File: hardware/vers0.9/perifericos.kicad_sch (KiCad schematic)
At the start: 27 parts, among them J4 Conn_02x13_Odd_Even, J5 Teclado, J6 Encoders, U10 ULN2803A, U2 74HC595, U6 74HC165

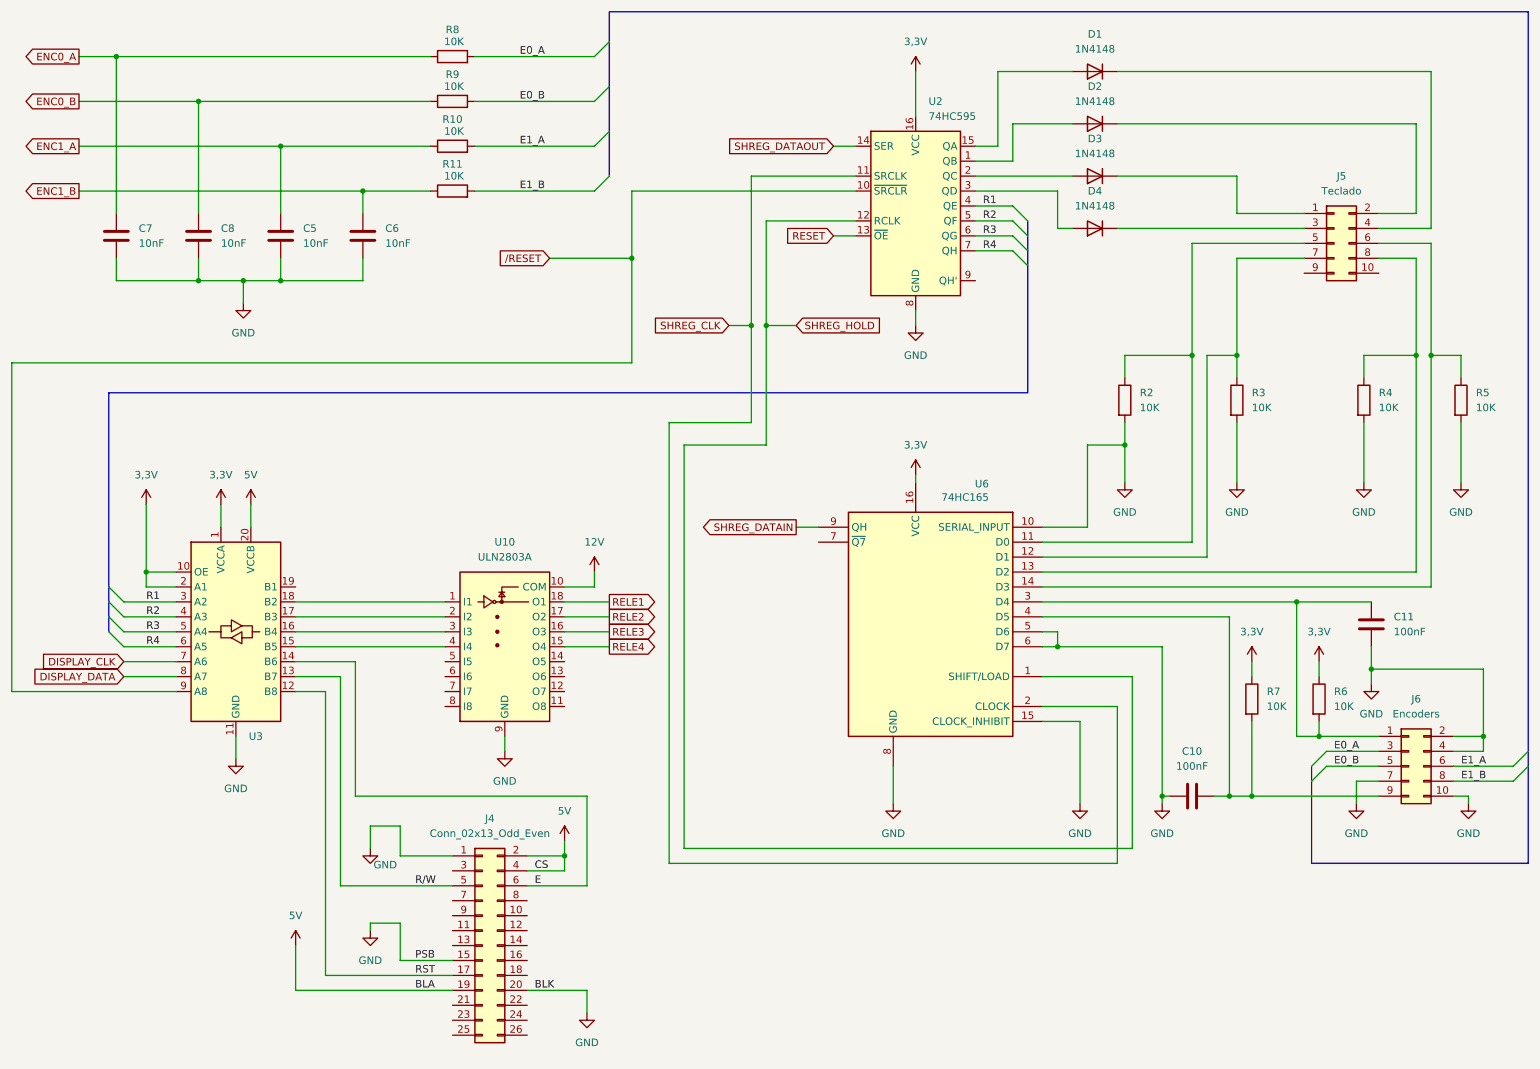
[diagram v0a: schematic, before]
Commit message: 250826-1410
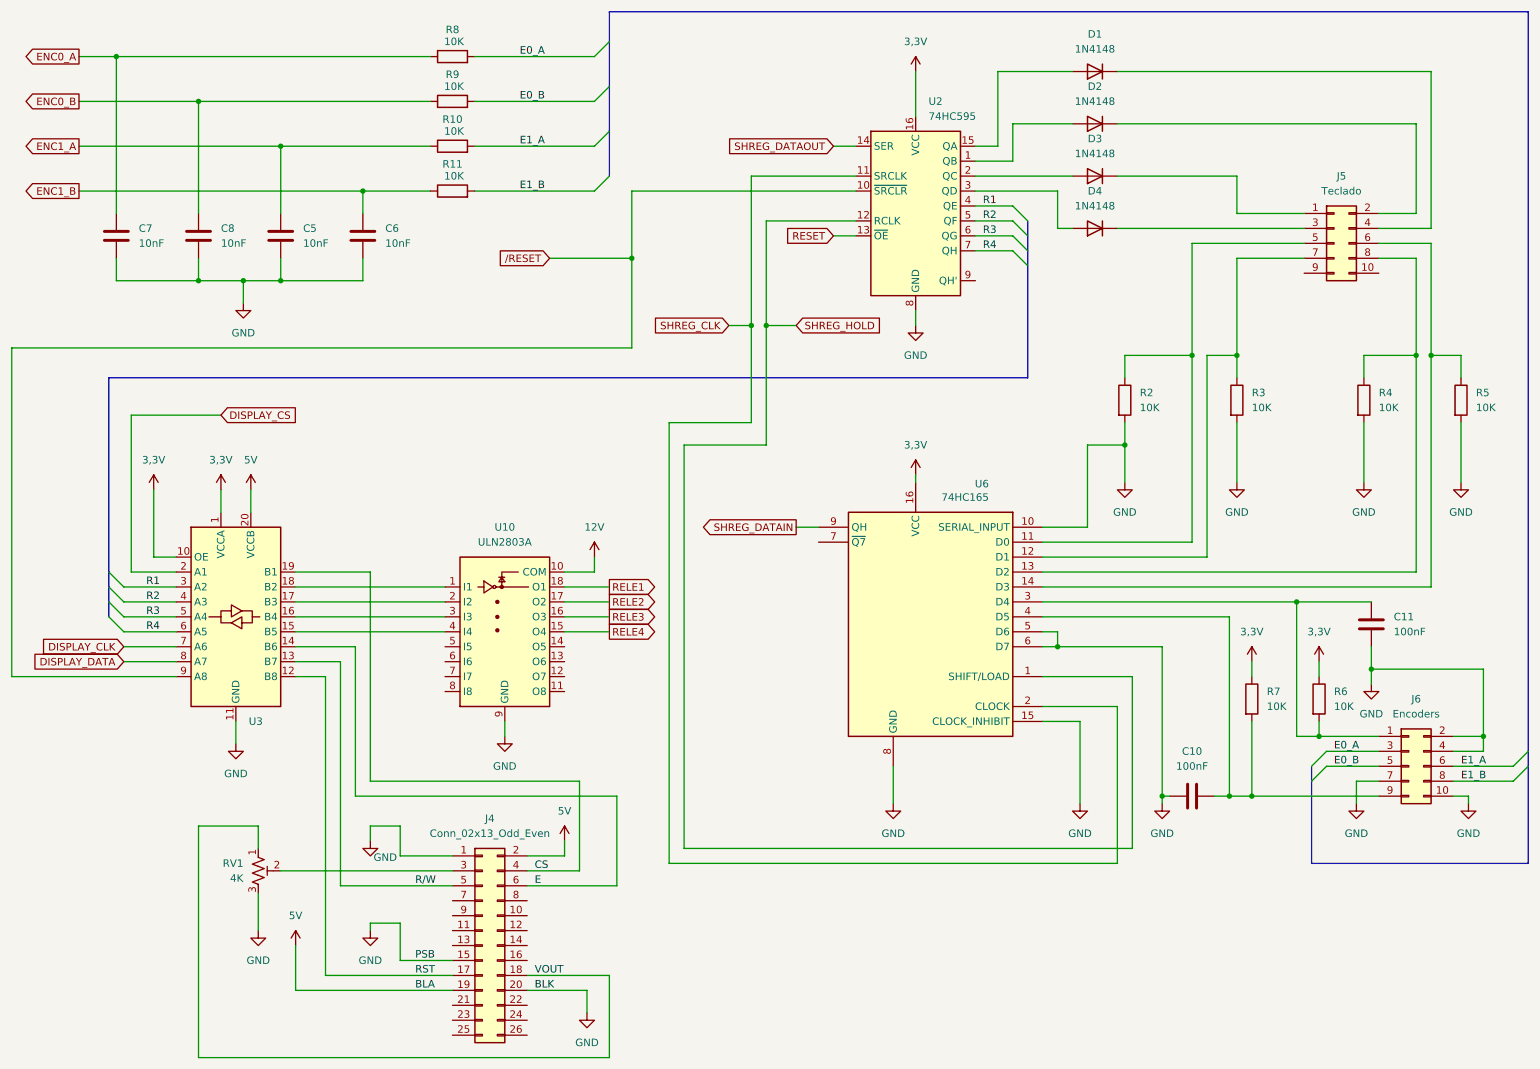
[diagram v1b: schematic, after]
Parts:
- added RV1: 4K, symbol Device:R_Potentiometer_Trim_US
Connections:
- net 3,3V: no longer U3.2 (A1)
- net 5V: no longer J4.4 (Pin_4)
- net GND: now also RV1.3
- net VOUT: now reaches J4.18 (Pin_18)
- net VOUT: now also RV1.1
- net at J4.3 (Pin_3): now also RV1.2
- net CS: now reaches U3.19 (B1)
- net CS: now also J4.4 (Pin_4)
- new net DISPLAY_CS: U3.2 (A1)
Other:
- moved on the sheet: U10, U3

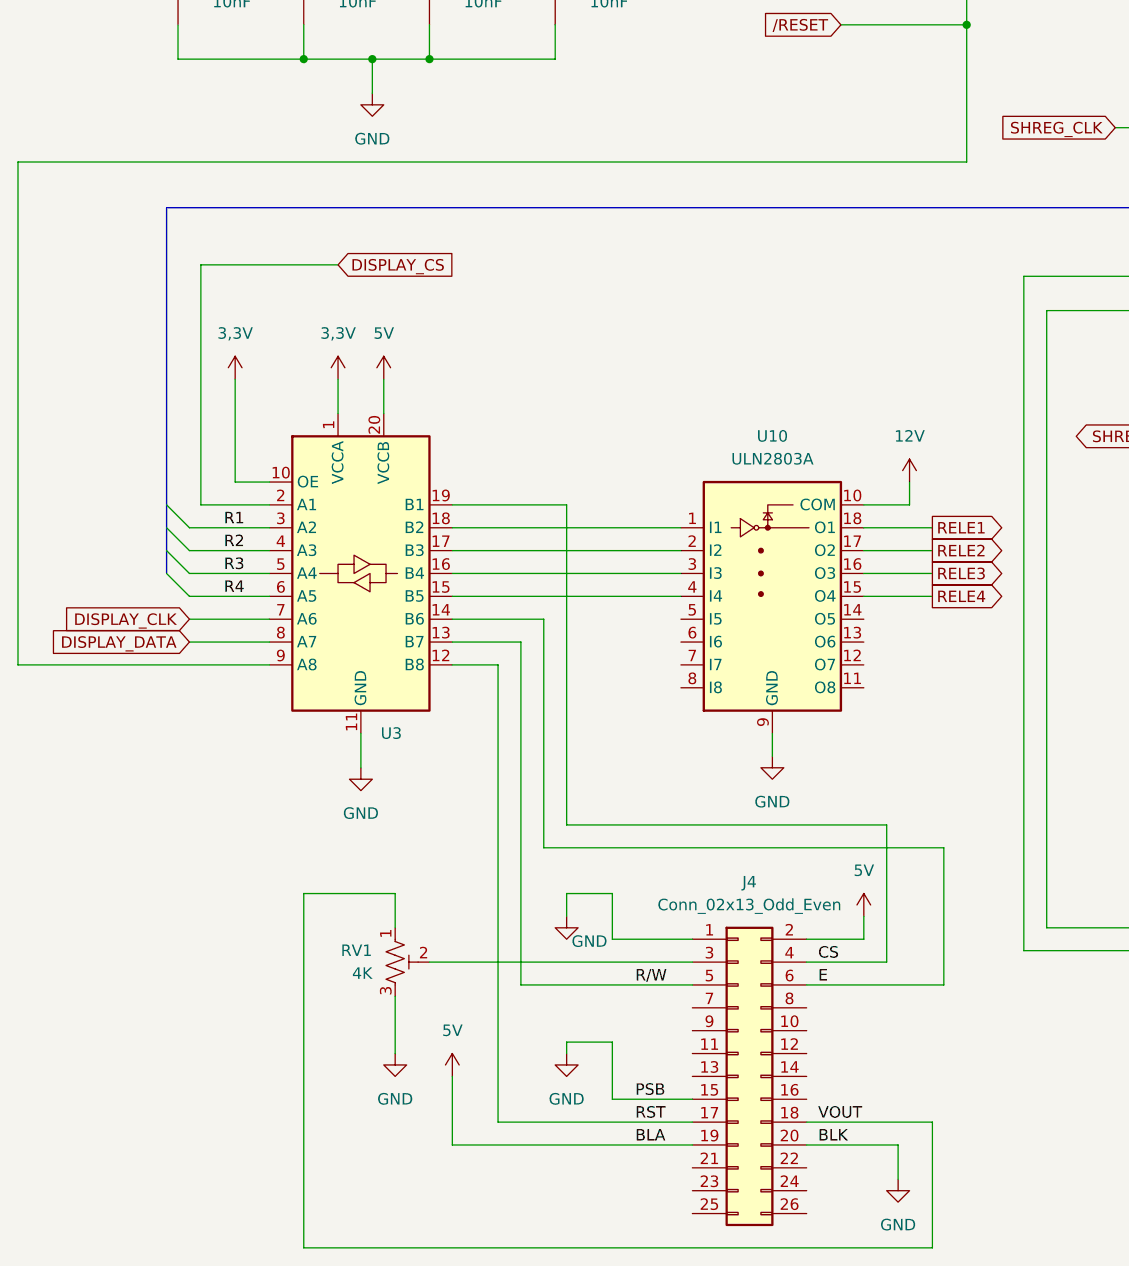
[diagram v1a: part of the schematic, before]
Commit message: 250827-1625
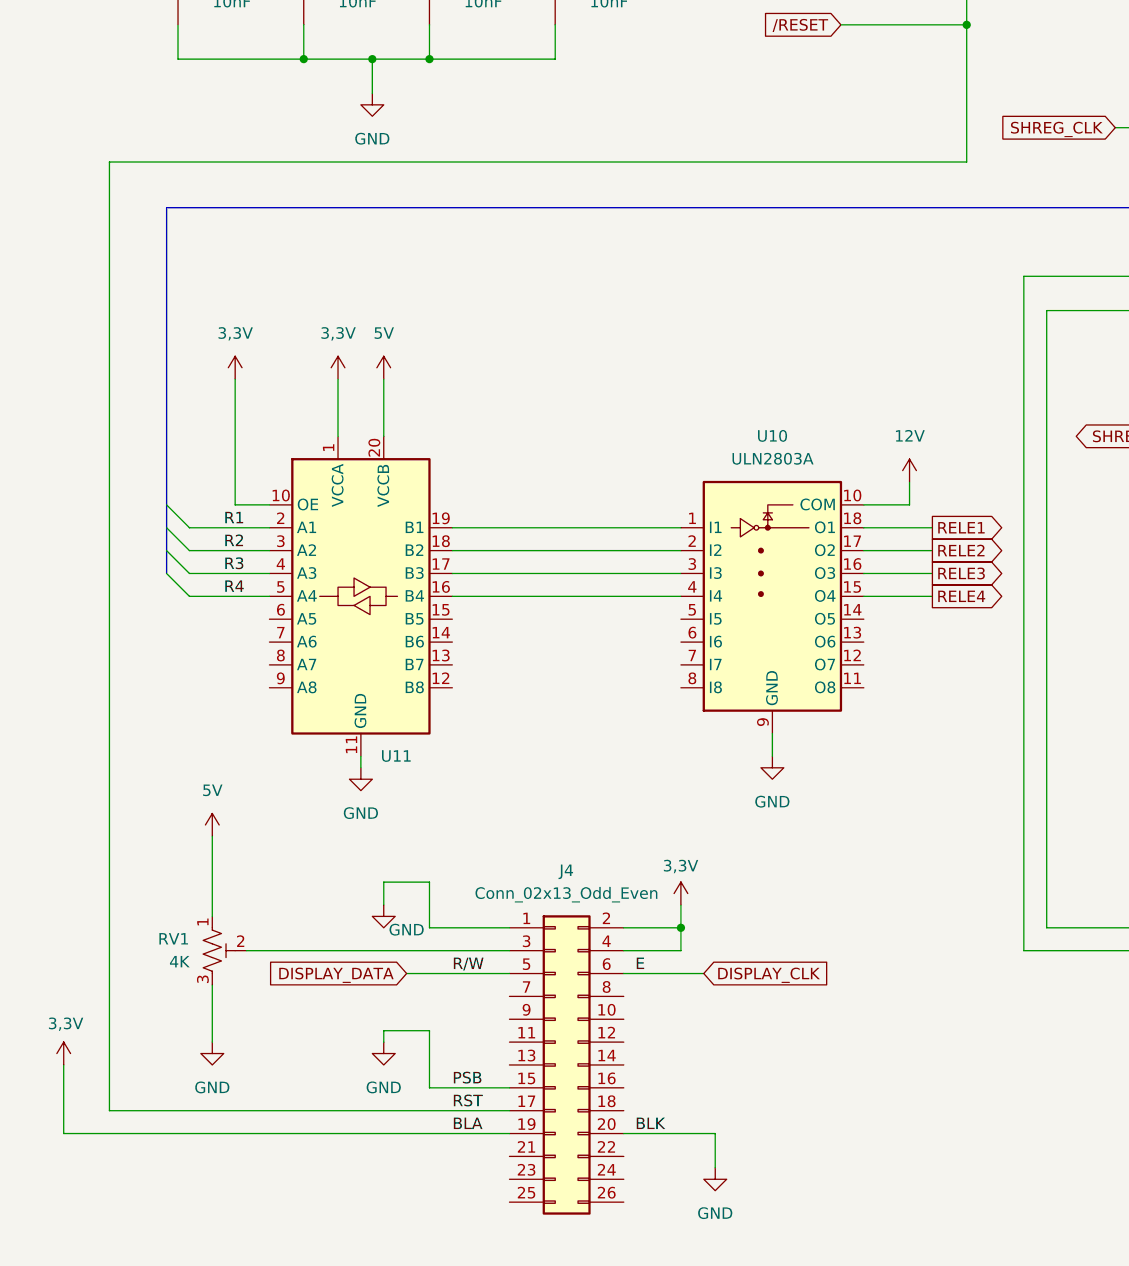
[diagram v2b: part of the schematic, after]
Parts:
- removed U3: ~, symbol dev_boards:TXB0108_BOARD
- added U11: ~, symbol dev_boards:TXB0108_BOARD
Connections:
- net CS is gone; now on net 3,3V: J4.4 (Pin_4)
- net E is gone; now on net DISPLAY_CLK: J4.6 (Pin_6)
- net RST is gone; now on net /RESET: J4.17 (Pin_17)
- net R/W is gone; now on net DISPLAY_DATA: J4.5 (Pin_5)
- net 3,3V: now also J4.19 (Pin_19), J4.2 (Pin_2), U11.1 (VCCA), U11.10 (OE)
- net 5V: now also RV1.1, U11.20 (VCCB); no longer J4.19 (Pin_19), J4.2 (Pin_2)
- net GND: now also U11.11 (GND)
- net R1: now also U11.2 (A1)
- net R2: now also U11.3 (A2)
- net R3: now also U11.4 (A3)
- net R4: now also U11.5 (A4)
- net at U10.4 (I4): now also U11.16 (B4)
- net at U10.3 (I3): now also U11.17 (B3)
- net at U10.2 (I2): now also U11.18 (B2)
- net at U10.1 (I1): now also U11.19 (B1)
- net VOUT: no longer names the net of J4.18 (Pin_18)
- net VOUT: no longer RV1.1
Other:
- moved on the sheet: J4, RV1
